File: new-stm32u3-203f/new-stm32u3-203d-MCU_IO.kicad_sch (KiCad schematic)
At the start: 8 parts, among them SW1 SW_SPDT, SW9 SW_RST, U1 STM32U385RGT6Q, X1 32.768kHz

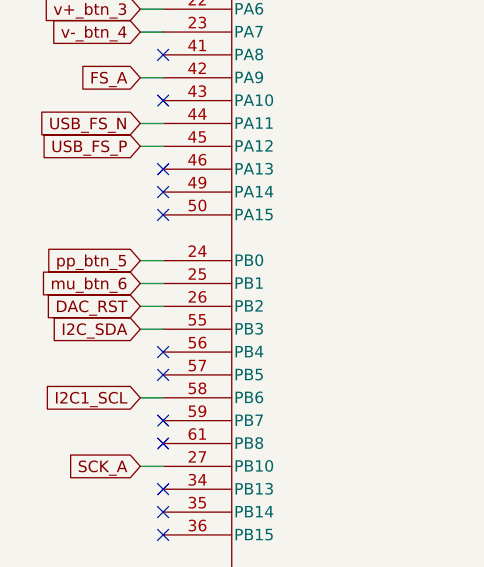
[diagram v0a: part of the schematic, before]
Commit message: made some progress on the pcb
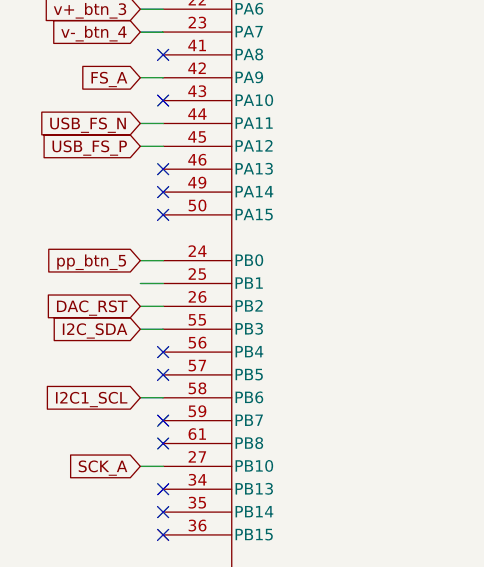
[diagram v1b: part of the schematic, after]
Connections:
- net mu_btn_6: no longer names the net of U1.25 (PB1)
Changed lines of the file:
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@@
-		)
-	)
-	(global_label "mu_btn_6"
-		(shape input)
-		(at 93.98 83.82 180)
-		(fields_autoplaced yes)
-		(effects
-			(font
-				(size 1.27 1.27)
-			)
-			(justify right)
-		)
-		(property "Intersheetrefs" "${INTERSHEET_REFS}"
-			(at 81.9841 83.82 0)
-			(effects
-				(font
-					(size 1.27 1.27)
-				)
-				(justify right)
-				(hide yes)
-			)
 		)
 	)
